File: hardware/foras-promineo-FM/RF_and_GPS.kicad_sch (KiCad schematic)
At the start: 15 parts, among them J12 Amphenol_901-144, J5 Amphenol_901-144, J6 Amphenol_901-144, J7 Amphenol_901-144, U13 EP2W+, U14 S1216V8, U15 RFM9xBreakout, U20 RFM9xBreakout, U23 RFM98PW, U24 RFM98PW

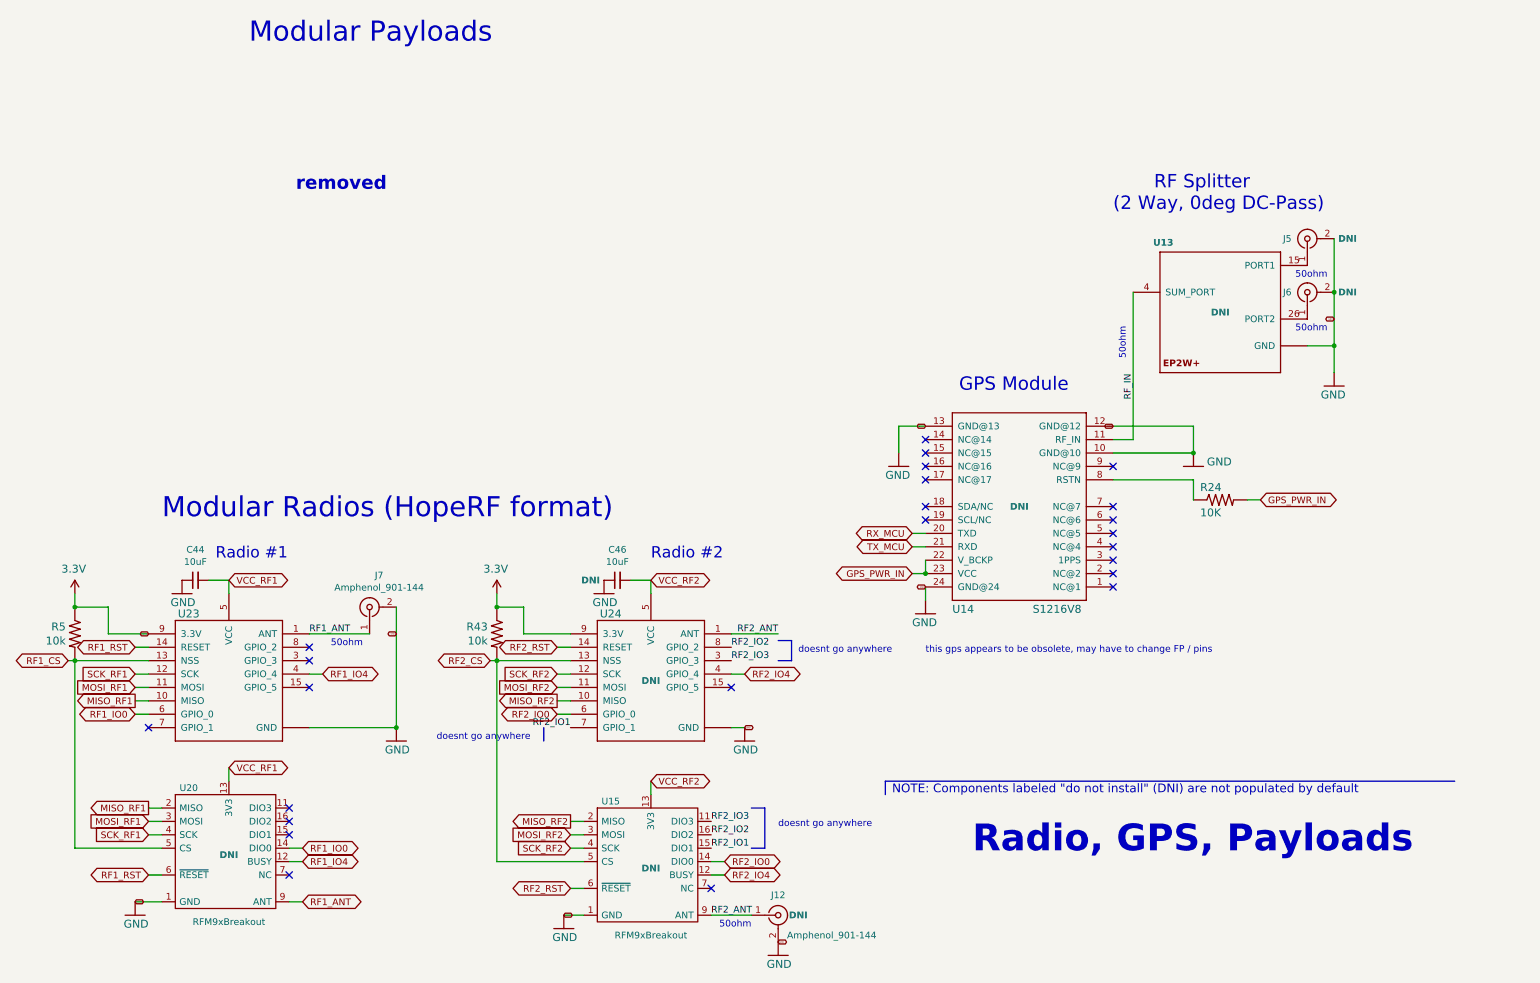
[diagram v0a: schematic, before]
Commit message: lots of stuff
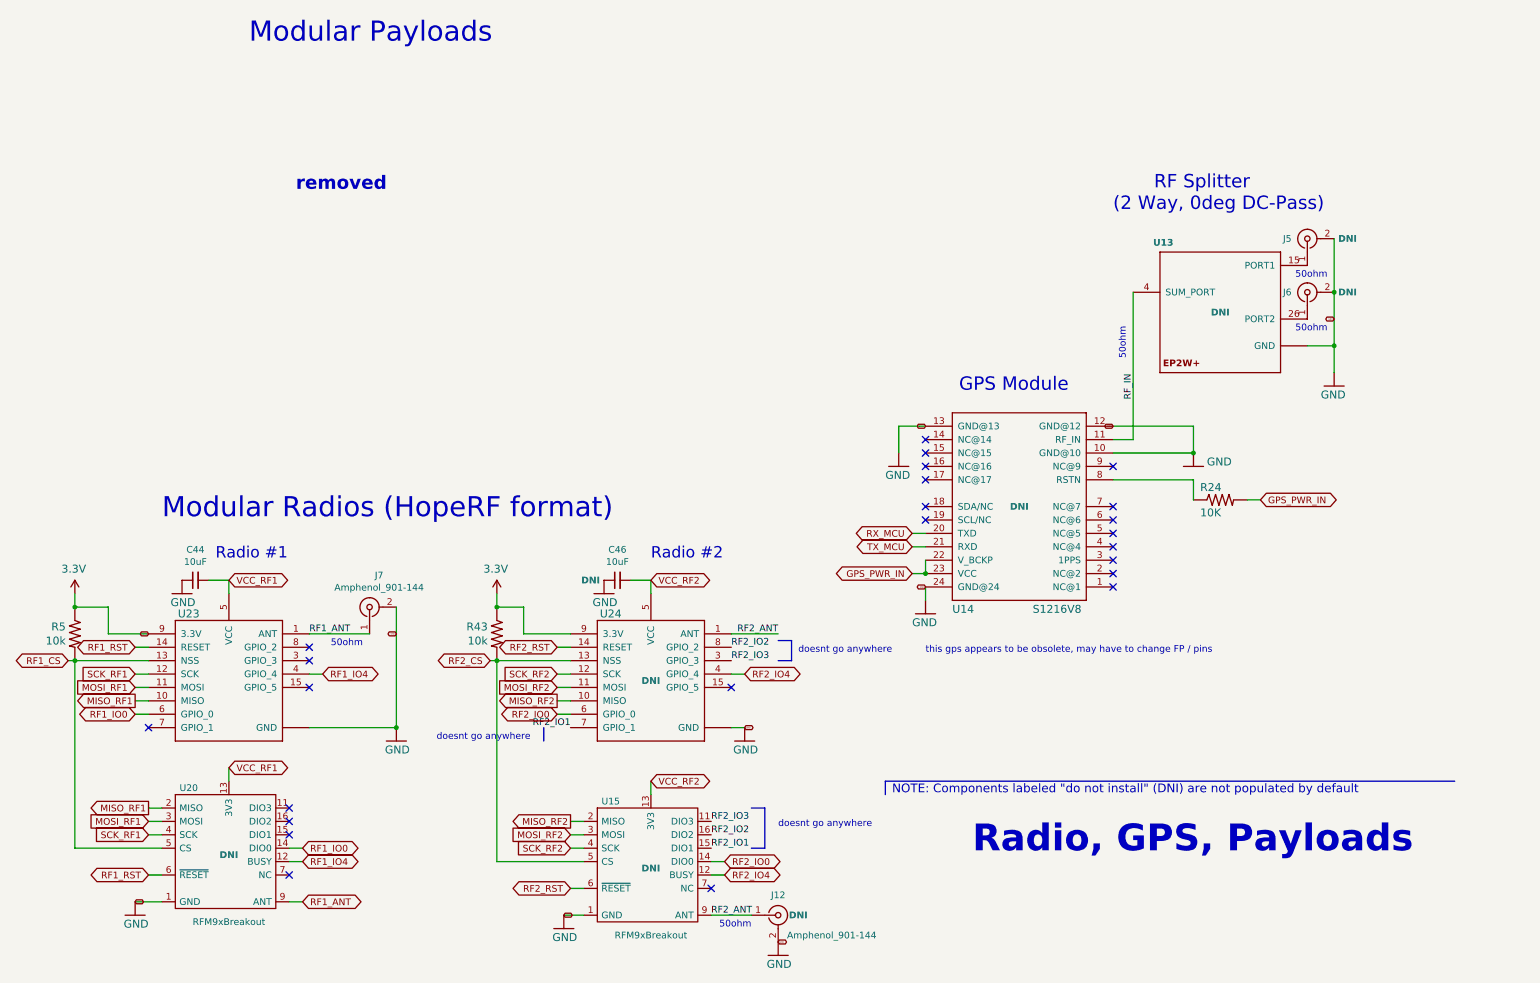
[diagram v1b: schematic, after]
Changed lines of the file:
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@@
     )
   )
-  (symbol (lib_id "mainboard:10KOHM-1_10W-1%(0603)0603") (at 240.03 109.22 0)
+  (symbol (lib_id "mainboard:10KOHM-1_10W-1%(0603)0603") (at 240.03 109.22 0) (unit 1)
     (in_bom yes) (on_board yes)
     (property "Reference" "R24" (id 0) (at 236.22 107.7214 0)
@@
     (pin "2")
   )
-  (symbol (lib_id "mainboard:GND") (at 261.62 87.63 0)
+  (symbol (lib_id "mainboard:GND") (at 261.62 87.63 0) (unit 1)
     (in_bom yes) (on_board yes)
     (property "Reference" "#GND044" (id 0) (at 261.62 87.63 0)
@@
     (pin "9")
   )
-  (symbol (lib_id "mainboard:GND") (at 83.82 154.94 0) (mirror y)
+  (symbol (lib_id "mainboard:GND") (at 83.82 154.94 0) (mirror y) (unit 1)
     (in_bom yes) (on_board yes)
     (property "Reference" "#GND0103" (id 0) (at 83.82 154.94 0)
@@
     (pin "2")
   )
-  (symbol (lib_id "mainboard:GND") (at 156.21 195.58 0) (mirror y)
+  (symbol (lib_id "mainboard:GND") (at 156.21 195.58 0) (mirror y) (unit 1)
     (in_bom yes) (on_board yes)
     (property "Reference" "#GND0105" (id 0) (at 156.21 195.58 0)
@@
     (pin "9")
   )
-  (symbol (lib_id "mainboard:GND") (at 115.57 190.5 0) (mirror y)
+  (symbol (lib_id "mainboard:GND") (at 115.57 190.5 0) (mirror y) (unit 1)
     (in_bom yes) (on_board yes)
     (property "Reference" "#GND0106" (id 0) (at 115.57 190.5 0)
@@
     (pin "1")
   )
-  (symbol (lib_id "mainboard:GND") (at 149.86 154.94 0) (mirror y)
+  (symbol (lib_id "mainboard:GND") (at 149.86 154.94 0) (mirror y) (unit 1)
     (in_bom yes) (on_board yes)
     (property "Reference" "#GND0107" (id 0) (at 149.86 154.94 0)
@@
     (pin "9")
   )
-  (symbol (lib_id "mainboard:GND") (at 34.29 187.96 0) (mirror y)
+  (symbol (lib_id "mainboard:GND") (at 34.29 187.96 0) (mirror y) (unit 1)
     (in_bom yes) (on_board yes)
     (property "Reference" "#GND0110" (id 0) (at 34.29 187.96 0)
@@
     (pin "1")
   )
-  (symbol (lib_id "mainboard:10KOHM-1_10W-1%(0603)0603") (at 102.87 134.62 270)
+  (symbol (lib_id "mainboard:10KOHM-1_10W-1%(0603)0603") (at 102.87 134.62 270) (unit 1)
     (in_bom yes) (on_board yes)
     (property "Reference" "R43" (id 0) (at 101.1428 133.2738 90)
@@
     (pin "2")
   )
-  (symbol (lib_id "mainboard:10KOHM-1_10W-1%(0603)0603") (at 22.86 134.62 270)
+  (symbol (lib_id "mainboard:10KOHM-1_10W-1%(0603)0603") (at 22.86 134.62 270) (unit 1)
     (in_bom yes) (on_board yes)
     (property "Reference" "R5" (id 0) (at 21.1328 133.2738 90)
@@
     (pin "2")
   )
-  (symbol (lib_id "mainboard:3.3V") (at 102.87 127 0)
+  (symbol (lib_id "mainboard:3.3V") (at 102.87 127 0) (unit 1)
     (in_bom yes) (on_board yes)
     (property "Reference" "#SUPPLY0104" (id 0) (at 102.87 127 0)
@@
     (pin "1")
   )
-  (symbol (lib_id "mainboard:3.3V") (at 22.86 127 0)
+  (symbol (lib_id "mainboard:3.3V") (at 22.86 127 0) (unit 1)
     (in_bom yes) (on_board yes)
     (property "Reference" "#SUPPLY0109" (id 0) (at 22.86 127 0)
@@
     (pin "1")
   )
-  (symbol (lib_id "mainboard-rescue:C_Small-Device-mainboard-rescue") (at 45.72 124.46 90)
+  (symbol (lib_id "mainboard-rescue:C_Small-Device-mainboard-rescue") (at 45.72 124.46 90) (unit 1)
     (in_bom yes) (on_board yes)
     (property "Reference" "C44" (id 0) (at 45.72 118.6434 90))
@@
     (pin "2")
   )
-  (symbol (lib_id "mainboard:GND") (at 43.18 127 0) (mirror y)
+  (symbol (lib_id "mainboard:GND") (at 43.18 127 0) (mirror y) (unit 1)
     (in_bom yes) (on_board yes)
     (property "Reference" "#GND036" (id 0) (at 43.18 127 0)
@@
     (pin "1")
   )
-  (symbol (lib_id "mainboard-rescue:C_Small-Device-mainboard-rescue") (at 125.73 124.46 90)
+  (symbol (lib_id "mainboard-rescue:C_Small-Device-mainboard-rescue") (at 125.73 124.46 90) (unit 1)
     (in_bom yes) (on_board yes)
     (property "Reference" "C46" (id 0) (at 125.73 118.6434 90))
@@
     (pin "2")
   )
-  (symbol (lib_id "mainboard:GND") (at 123.19 127 0) (mirror y)
+  (symbol (lib_id "mainboard:GND") (at 123.19 127 0) (mirror y) (unit 1)
     (in_bom yes) (on_board yes)
     (property "Reference" "#GND038" (id 0) (at 123.19 127 0)
@@
     (pin "1")
   )
-  (symbol (lib_id "mainboard:EP2W+") (at 241.3 69.85 0)
+  (symbol (lib_id "mainboard:EP2W+") (at 241.3 69.85 0) (unit 1)
     (in_bom yes) (on_board yes)
     (property "Reference" "U13" (id 0) (at 231.14 59.69 0)
@@
     (pin "EP")
   )
-  (symbol (lib_id "mainboard:GND") (at 179.07 102.87 0)
+  (symbol (lib_id "mainboard:GND") (at 179.07 102.87 0) (unit 1)
     (in_bom yes) (on_board yes)
     (property "Reference" "#GND042" (id 0) (at 179.07 102.87 0)
@@
     (pin "1")
   )
-  (symbol (lib_id "mainboard:GND") (at 184.15 130.81 0)
+  (symbol (lib_id "mainboard:GND") (at 184.15 130.81 0) (unit 1)
     (in_bom yes) (on_board yes)
     (property "Reference" "#GND043" (id 0) (at 184.15 130.81 0)
@@
     (pin "1")
   )
-  (symbol (lib_id "mainboard:GND") (at 234.95 102.87 0)
+  (symbol (lib_id "mainboard:GND") (at 234.95 102.87 0) (unit 1)
     (in_bom yes) (on_board yes)
     (property "Reference" "#GND047" (id 0) (at 234.95 102.87 0)
@@
     (pin "1")
   )
-  (symbol (lib_id "mainboard:S1216V8") (at 201.93 110.49 0)
+  (symbol (lib_id "mainboard:S1216V8") (at 201.93 110.49 0) (unit 1)
     (in_bom yes) (on_board yes)
     (property "Reference" "U14" (id 0) (at 189.23 130.81 0)
